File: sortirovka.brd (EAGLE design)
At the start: 79.4 x 80.9 mm, 44 parts, among them IC1 DS1307Z, U1 MAX3485CSA, X1 PI3-CON, X2 MKDSN1,5/2-5,08, X3 MKDSN1,5/4-5,08, X4 MKDSN1,5/2-5,08, X6 22-23-2051, X7 22-23-2041, X8 22-23-2051, X9 MKDSN1,5/7-5,08

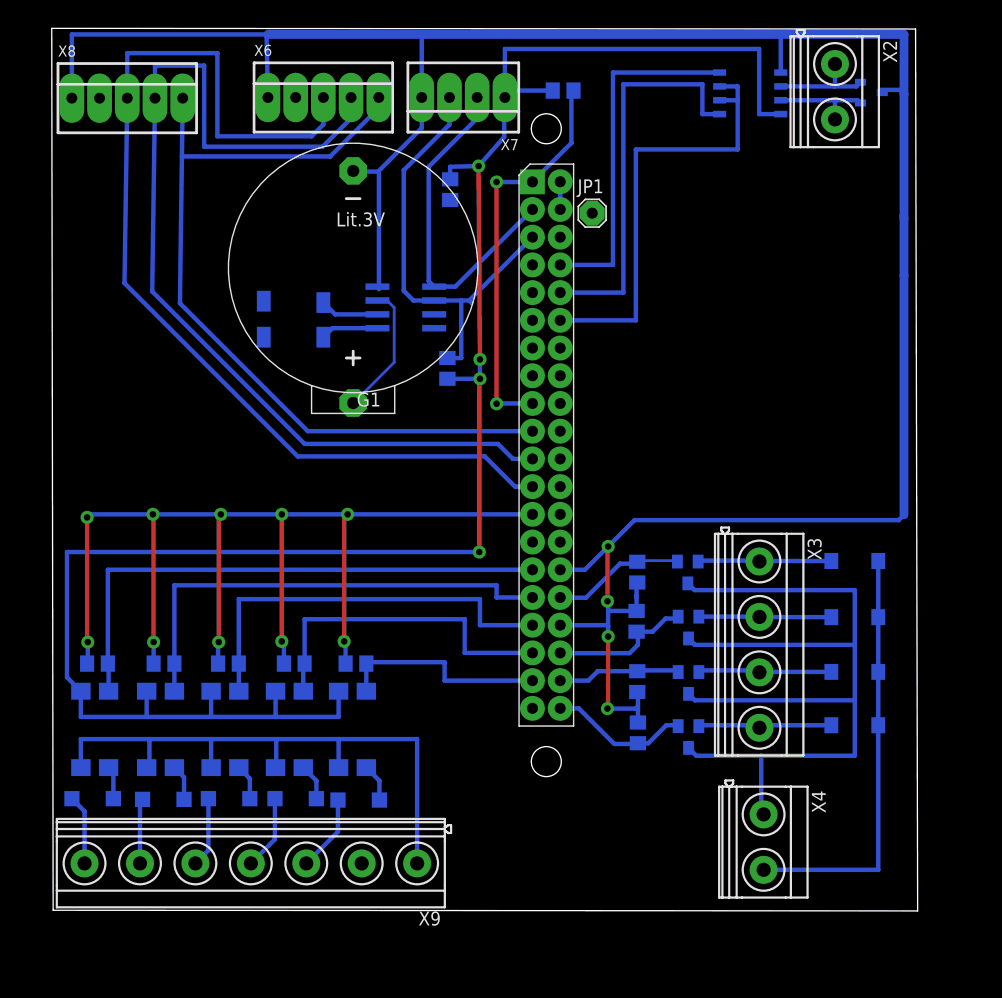
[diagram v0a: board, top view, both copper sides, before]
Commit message: rev1.0 to produce
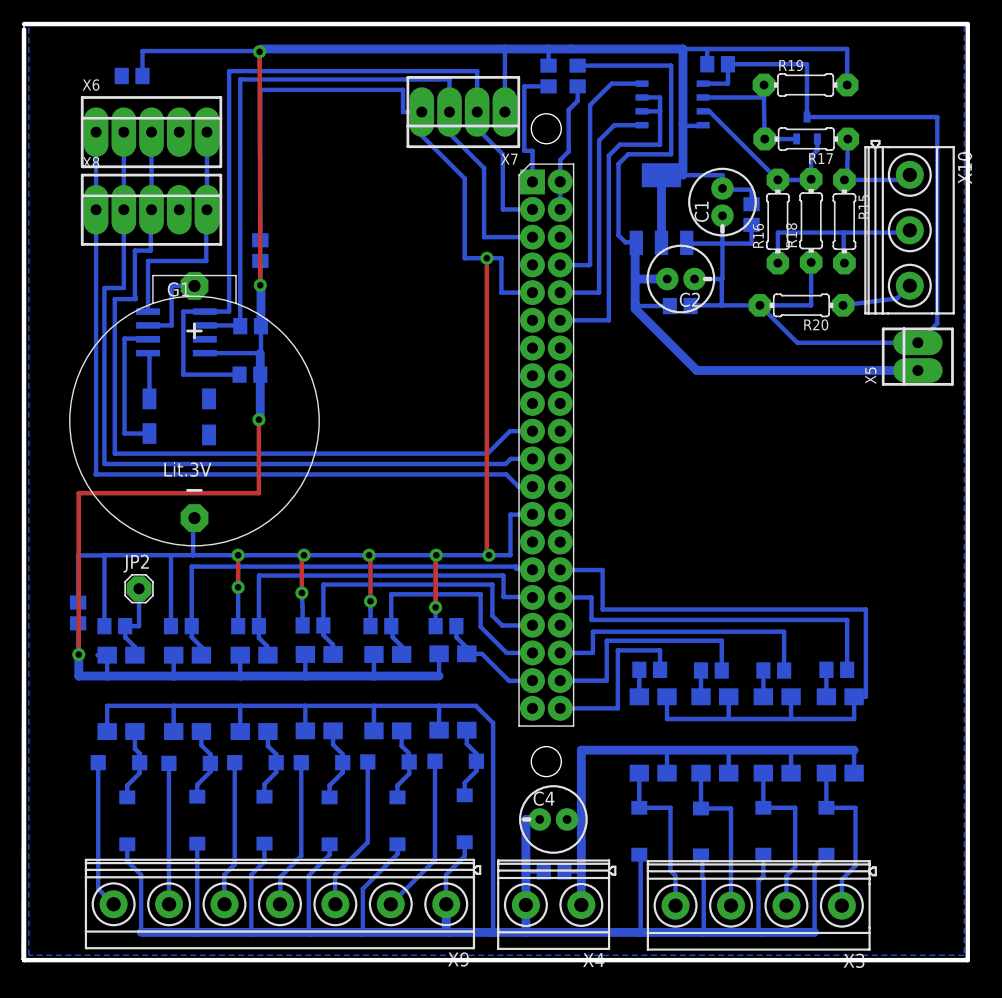
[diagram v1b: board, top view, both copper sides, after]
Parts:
- removed JP1: (no value), pinhead:1X01
- removed Q1, Q2, Q3, Q4: (no value), MyLib:SOT23-WIDE
- removed X2: MKDSN1,5/2-5,08, con-phoenix-508:MKDSN1,5/2-5,08
- added C1, C2, C4: (no value), rcl:SANYO-OSCON_C
- added C10, C3, C5, C6, C7, C8, C9: 0.1, rcl:C0805
- added D10, D5, D6, D7, D8, D9: DIODE1N4007, MyLib:SMA-DIODE
- added IC3: LM1117IMPX-3.3, lm1117:SOT223
- added JP2: (no value), pinhead:1X01
- added OC10, OC6, OC7, OC8, OC9: (no value), MyLib:SMD4
- added R13: 10k, rcl:R0805
- added R14: 0, rcl:R0805
- added R15: 120, rcl:0204/7
- added R16, R17: 47, rcl:0204/7
- added R18, R19, R20: 560, rcl:0204/7
- added U$7: NSI45020AT1GSOD-123, MyLib:SOD123
- added X10: MKDSN1,5/3-5,08, con-phoenix-508:MKDSN1,5/3-5,08
- added X5: 22-23-2021, con-molex:22-23-2021
- R1, R2, R3, R4: value 10k -> 200
- moved R11 25.0 mm to (18.3, 49.1), turned to 180 degrees
- moved D4 24.9 mm to (71.1, 7.30), turned to 90 degrees
- moved X3 23.9 mm to (64.9, 0.51), turned to 180 degrees
- moved D3 22.0 mm to (54.0, 7.30), turned to 90 degrees
- moved D1 21.3 mm to (65.3, 7.30), turned to 90 degrees
- moved IC1 21.1 mm to (11.6, 53.0)
- moved R4 20.4 mm to (72.1, 22.1), turned to 180 degrees
- moved D2 20.3 mm to (59.6, 7.24), turned to 90 degrees
- moved G1 20.2 mm to (13.2, 44.9), turned to 0 degrees
- moved X4 20.1 mm to (46.1, 0.57), turned to 180 degrees
- moved R10 18.4 mm to (18.4, 53.6), turned to 180 degrees
- moved X6 16.1 mm to (9.27, 71.4)
- moved Q5 13.6 mm to (11.6, 45.7), turned to 180 degrees
- moved R3 13.4 mm to (66.3, 22.0), turned to 180 degrees
- moved X8 10.5 mm to (9.27, 64.3)
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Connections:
- removed net +5V: IC1.8
- removed net N$31: OC5.4, R12.2, X1.P$37
- new net N$34: OC6.4, R13.2, X1.P$37
- new net N$36: D10.C, OC6.1, U$7.C
- new net N$38: U$7.A, X9.2
- new net N$39: OC5.4, R12.2, X1.P$35
- new net N$40: OC4.4, R9.2, X1.P$33
- new net N$41: OC3.4, R8.2, X1.P$31
- new net N$42: OC2.4, R6.2, X1.P$29
- new net N$43: JP2.1, OC1.4, R5.2, X1.P$7
- new net N$45: R15.2, R16.1, X10.2
- new net N$46: R15.1, R17.1, X10.1
- new net N$47: R17.2, R19.1, U$3.2, U1.6
- new net PW: C2.+, C3.1, IC3.3, R14.2, X5.1
- net +24V: now also C4.+, C6.1, OC10.3, OC7.3, OC8.3, OC9.3; no longer Q1.3, Q2.3, Q3.3, Q4.3
- net +3V3: now also C1.+, C10.1, C5.1, C7.1, C8.1, C9.1, IC1.8, IC3.2, IC3.TAB, OC6.3, R19.2
- net GND: now also C1.-, C10.2, C2.-, C3.2, C5.2, C7.2, C8.2, C9.2, IC3.1, OC10.2, OC7.2, OC8.2, OC9.2, R13.1, R18.1, R20.2, X5.2, X6.5, X8.5; no longer R1.1, R2.1, R3.1, R4.1, X6.1, X8.1
- net GND1: now also C4.-, C6.2, D10.A, D5.A, D6.A, D7.A, D8.A, D9.A, OC6.2
- net MISO: now also X6.2, X8.2; no longer X6.4, X8.4
- net MOSI: now also X6.3, X8.3; no longer X6.5, X8.5
- net N$10: now also OC10.4; no longer Q4.2
- net N$11: now also OC9.4; no longer Q3.2
- net N$12: now also OC8.4; no longer Q2.2
- net N$13: now also OC7.4; no longer Q1.2
- net N$15: now also OC7.1, R1.1; no longer OC2.4, R6.2, X1.P$31
- net N$16: now also D5.C
- net N$17: now also D6.C
- net N$18: now also OC8.1, R2.1; no longer OC1.4, R5.2, X1.P$29
- net N$19: now also OC9.1, R3.1; no longer OC3.4, R8.2, X1.P$33
- net N$24: now also D7.C
- net N$28: now also R14.1; no longer JP1.1
- net N$29: now also OC10.1, R4.1; no longer OC4.4, R9.2, X1.P$35
- net N$30: now also D8.C
- net N$32: now also D9.C
- net N$4: now also R16.2, R18.2, U$3.1, U1.7; no longer U$3.2, U1.6, X2.1
- net N$5: now also R20.1, X10.3; no longer U$3.1, U1.7, X2.2
- net N$6: no longer Q1.1
- net N$7: no longer Q2.1
- net N$8: no longer Q3.1
- net N$9: no longer Q4.1
- net SPI0: now also X6.4; no longer X6.2
- net SPI1: now also X8.4; no longer X8.2
- net SPI_CLK: now also X6.1, X8.1; no longer X6.3, X8.3
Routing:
- net GND1: track 94.4 -> 227.5 mm
- net PW: track 0.00 -> 70.9 mm
- net +3V3: track 176.2 -> 239.9 mm
- net N$18: track 50.1 -> 2.41 mm
- net N$27: track 31.6 -> 76.3 mm
- net N$15: track 43.6 -> 2.47 mm
- net N$42: track 0.00 -> 40.0 mm
- net N$19: track 37.7 -> 2.41 mm
- net N$41: track 0.00 -> 34.7 mm
- net +24V: track 82.8 -> 50.8 mm
- net N$40: track 0.00 -> 29.2 mm
- net N$29: track 30.7 -> 2.47 mm
- net N$14: track 37.1 -> 11.7 mm, vias 2 -> 0
- net N$26: track 40.9 -> 65.2 mm
- net N$39: track 0.00 -> 23.0 mm
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- added copper zone on layer 16, net GND
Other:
- board size 79.4 x 80.9 mm -> 86.8 x 85.8 mm
